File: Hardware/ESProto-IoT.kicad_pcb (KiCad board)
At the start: 2 copper layers, 68.6 x 53.3 mm, 55 parts, among them IC1 ARDUINO_PRO_MINI_5V, P1 DIGITAL_02, P10 DIGITAL_11, P11 DIGITAL_12, P12 DIGITAL_13X, P13 ANALOG_00, P14 ANALOG_01, P15 ANALOG_02, P16 ANALOG_03X, P17 I2C_01, P18 I2C_02, P19 I2C_03, P2 DIGITAL_03, P20 I2C_04, P21 POWER_L, P22 POWER_R, P23 ESP_G14, P24 ESP_G12, P25 ESP_G13, P26 ESP_3V3, P27 ESP_RST, P28 ESP_ADC, P29 ESP_G16, P3 DIGITAL_04, P30 LEVEL_T1, P31 LEVEL_B3, P32 ESP_TX, P33 ESP_RX, P34 ESP_G5, P35 ESP_G4, P36 LEVEL_B2, P37 LEVEL_B1, P38 ESP_G0, P39 ESP_G2, P4 DIGITAL_05, P40 ESP_G15, P41 ESP_GND, P42 ARDUINO_L, P43 I2C_A4_A5, P44 ARDUINO_R, P45 J_RAW_5V, P5 DIGITAL_06, P6 DIGITAL_07, P7 DIGITAL_08, P8 DIGITAL_09, P9 DIGITAL_10, SW1 PROGRAM

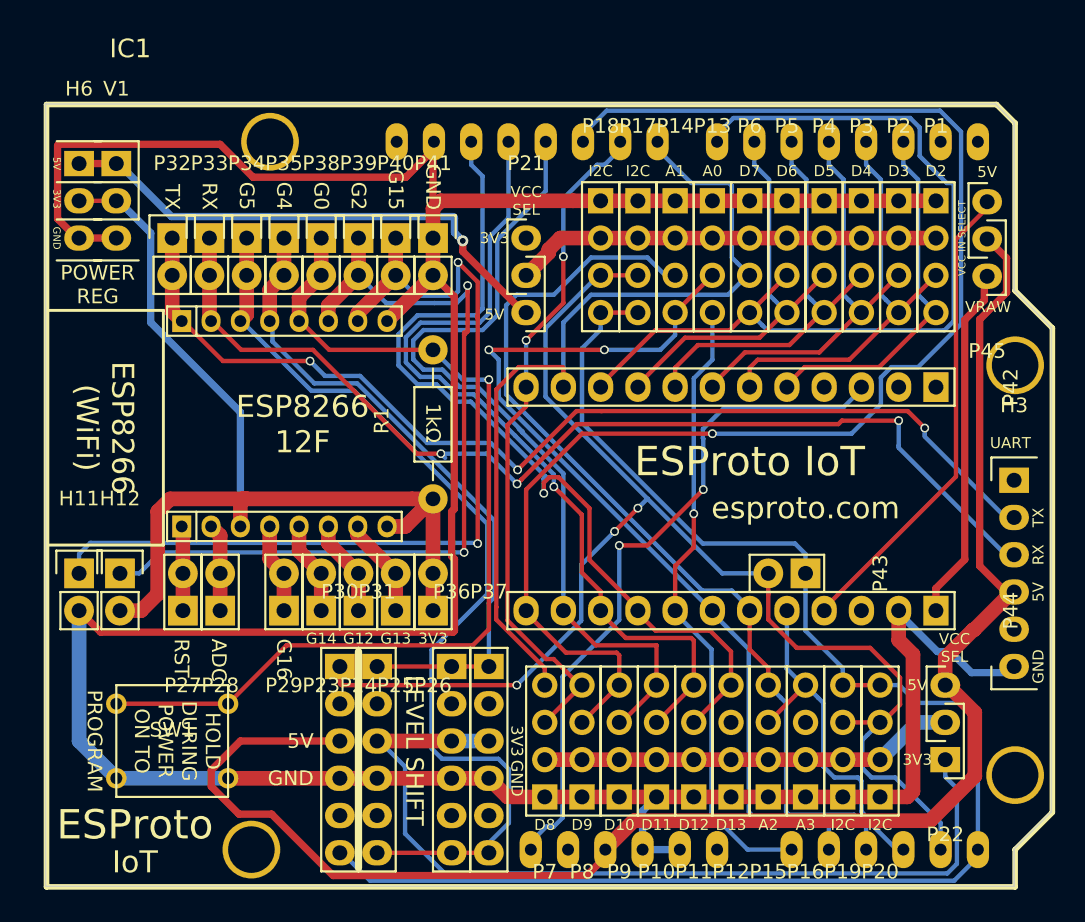
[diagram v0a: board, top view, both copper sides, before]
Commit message: Update to v20160308
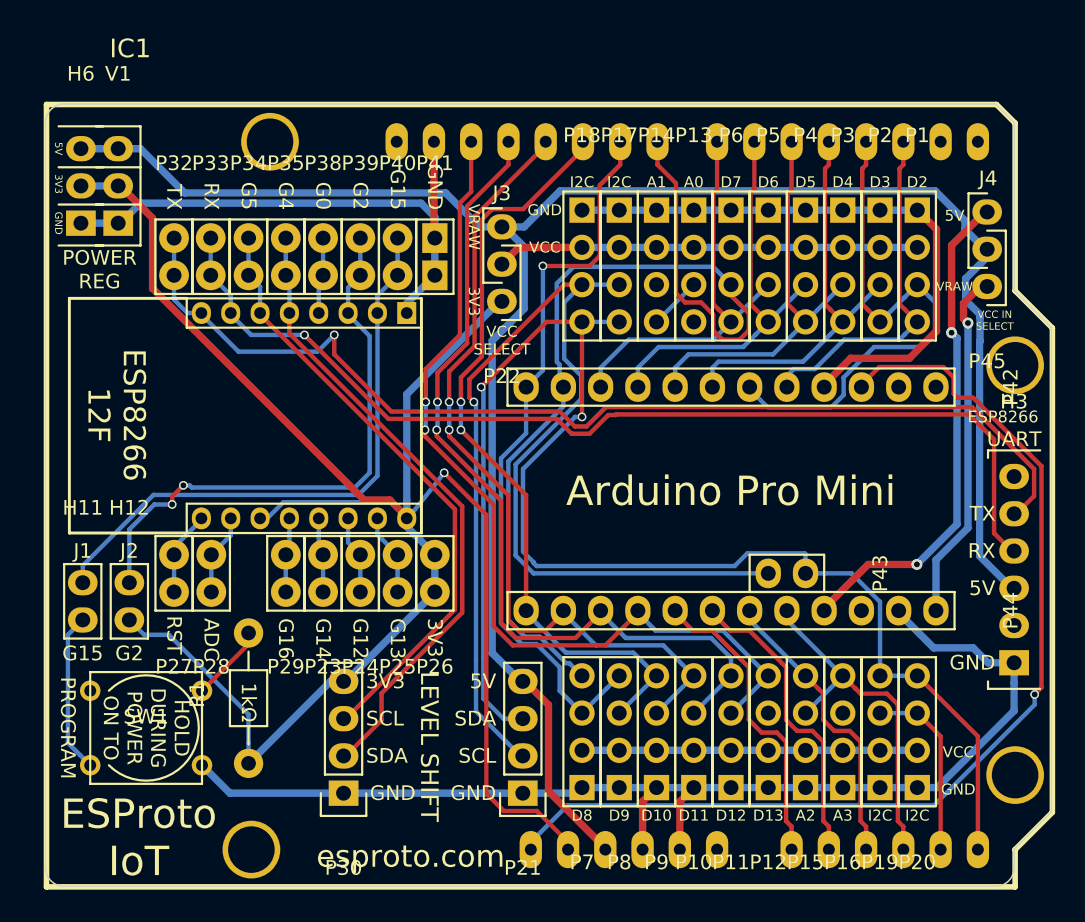
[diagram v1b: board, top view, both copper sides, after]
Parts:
- removed P31: LEVEL_B3, Pin_Headers:Pin_Header_Straight_1x06
- removed P36: LEVEL_B2, Pin_Headers:Pin_Header_Straight_1x06
- removed P37: LEVEL_B1, Pin_Headers:Pin_Header_Straight_1x06
- P21: value POWER_L -> LEVEL_A; footprint Pin_Headers:Pin_Header_Straight_1x03 -> Pin_Headers:Pin_Header_Straight_1x04
- P22: value POWER_R -> POWER_A
- P30: value LEVEL_T1 -> LEVEL_B; footprint Pin_Headers:Pin_Header_Straight_1x06 -> Pin_Headers:Pin_Header_Straight_1x04
- moved P22 43.5 mm to (124.1, 56.4)
- moved P21 37.8 mm to (125.5, 89.9), turned to 180 degrees
- moved R1 22.5 mm to (106.8, 83.4)
- moved P30 8.64 mm to (113.3, 89.9), turned to 180 degrees
- moved P12 2.62 mm to (142.2, 89.5)
- moved P19 2.62 mm to (149.9, 89.5)
- moved P8 2.62 mm to (132.1, 89.5)
- moved P10 2.62 mm to (137.2, 89.5)
- moved P11 2.62 mm to (139.7, 89.5)
- moved P15 2.62 mm to (144.8, 89.5)
- moved P16 2.62 mm to (147.3, 89.5)
- moved P20 2.62 mm to (152.4, 89.5)
- moved P7 2.62 mm to (129.5, 89.5)
- moved P9 2.62 mm to (134.6, 89.5)
- moved SW1 1.99 mm to (99.8, 85.5)
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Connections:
- P10 pad 2: Net-(P10-Pad2) -> Net-(P1-Pad2)
- P11 pad 2: Net-(P10-Pad2) -> Net-(P1-Pad2)
- P12 pad 2: Net-(P10-Pad2) -> Net-(P1-Pad2)
- P15 pad 2: Net-(P10-Pad2) -> Net-(P1-Pad2)
- P16 pad 2: Net-(P10-Pad2) -> Net-(P1-Pad2)
- P19 pad 2: Net-(P10-Pad2) -> Net-(P1-Pad2)
- P20 pad 2: Net-(P10-Pad2) -> Net-(P1-Pad2)
- P21 pad 1: +3V3 -> GND
- P21 pad 2: Net-(P1-Pad2) -> SDA
- P21 pad 3: +5V -> SCL
- P22 pad 2: Net-(P10-Pad2) -> Net-(P1-Pad2)
- P30 pad 1: SDA -> GND
- P30 pad 2: Net-(P30-Pad2) -> SDA_ESP
- P30 pad 3: +5V -> SCL_ESP
- P30 pad 4: GND -> +3V3
- P7 pad 2: Net-(P10-Pad2) -> Net-(P1-Pad2)
- P8 pad 2: Net-(P10-Pad2) -> Net-(P1-Pad2)
- P9 pad 2: Net-(P10-Pad2) -> Net-(P1-Pad2)
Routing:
- net GND: track 239.6 -> 172.1 mm
- net GPIO0: track 65.4 -> 10.5 mm, vias 1 -> 0
- net D10: track 97.6 -> 52.9 mm, vias 1 -> 2
- net A2: track 64.5 -> 20.2 mm
- net A1: track 64.5 -> 24.6 mm, vias 2 -> 0
- net D7: track 60.1 -> 28.0 mm
- net Net-(P10-Pad2): track 28.4 -> 0.00 mm
- net RST2: track 47.1 -> 71.7 mm, vias 2 -> 1
- net SCL_ESP: track 65.2 -> 41.8 mm
- net Net-(P1-Pad2): track 29.1 -> 51.7 mm
- net GPIO15: track 62.5 -> 40.7 mm, vias 2 -> 0
- net A0: track 42.7 -> 21.0 mm, vias 1 -> 0
- net GPIO2: track 58.1 -> 39.1 mm
- net +5V: track 147.2 -> 139.8 mm, vias 1 -> 0
- net D3: track 29.2 -> 36.3 mm
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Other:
- outline, holes or cut-outs redrawn
- board text added: "Arduino Pro Mini"
- board text added: "ESP8266"
- board text added: "HOLD DURING POWER ON TO"
- board text added: "J1"
- board text added: "J2"
- board text added: "J3"
- board text added: "J4"
- board text added: "PROGRAM"
- board text added: "SCL"
- board text added: "SDA"
- board text added: "VCC"
- board text added: "VCC SELECT"
- board text added: "Version 20160308"
- board text removed: "ESP8266 (WiFi)"
- board text removed: "ESProto"
- board text removed: "HOLD DURING POWER ON TO PROGRAM"
- board text removed: "IoT"
- board text removed: "VCC SEL"
